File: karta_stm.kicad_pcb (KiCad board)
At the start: 2 copper layers, 99.1 x 63.5 mm, 130 parts, among them J1 Screw_Terminal_01x05, J2 Conn_01x06_Male, J3 Screw_Terminal_01x02, J4 Screw_Terminal_01x02, J5 Screw_Terminal_01x05, J6 Screw_Terminal_01x04, J7 Screw_Terminal_01x03, Q1 BC817, Q10 BC817, Q11 Q_PMOS_DGS, Q12 Q_NMOS_DGS, Q13 BC817, Q14 Q_PMOS_DGS, Q15 Q_NMOS_DGS, Q2 Q_PMOS_DGS, Q3 Q_NMOS_DGS, Q4 BC817, Q5 Q_PMOS_DGS, Q6 Q_NMOS_DGS, Q7 BC817, Q8 Q_PMOS_DGS, Q9 Q_NMOS_DGS, SW1 SW_Push, U1 STM32L4P5RET6, U10 EL817, U11 EL817, U12 EL817, U13 EL817, U2 MCP2562-H-SN, U3 LM2596S-5, U4 LD1117S33TR_SOT223, U5 MCP6001x-LT, U6 MCP6001x-LT, U7 MCP6001x-LT, U8 MCP6001x-LT, U9 MCP6001x-LT, Y1 16MHz

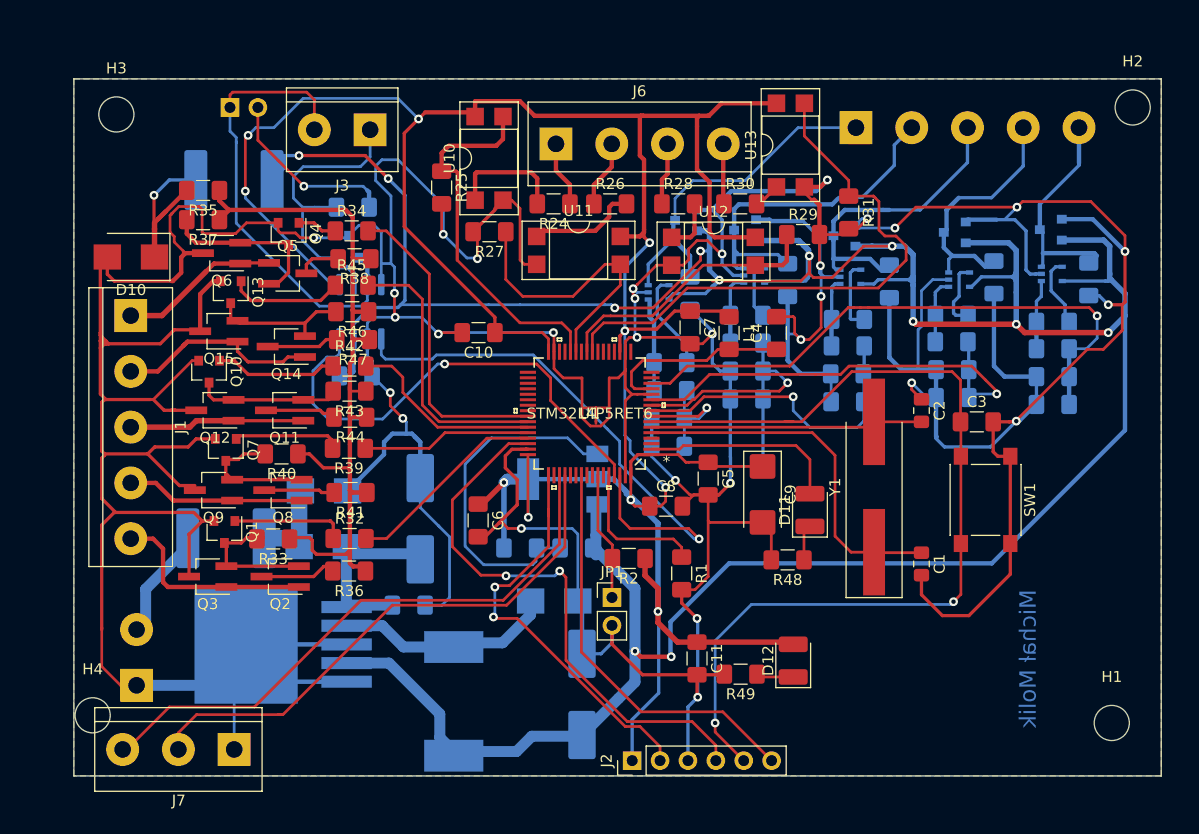
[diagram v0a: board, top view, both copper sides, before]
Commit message: Add files via upload
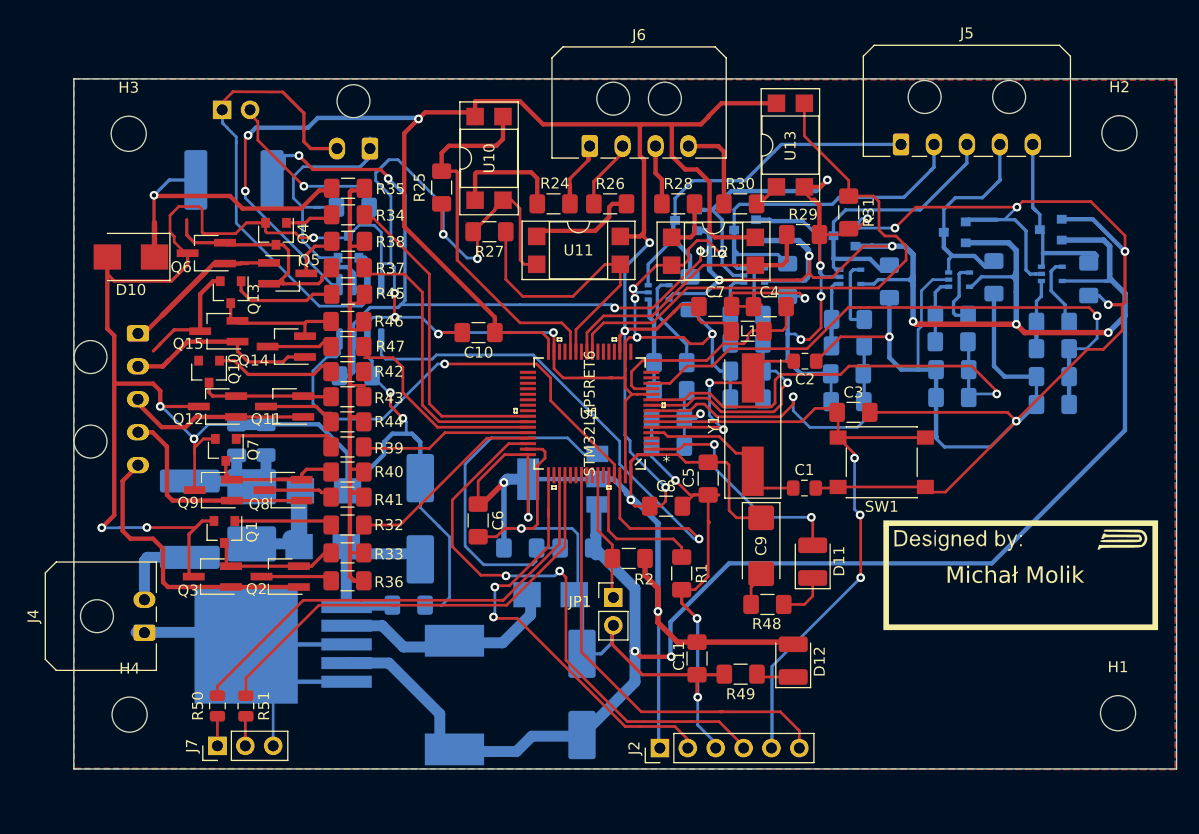
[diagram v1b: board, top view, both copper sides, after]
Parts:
- added C23: C, Capacitor_SMD:C_1206_3216Metric, B.Cu at (106.4, 84.9)
- added C24: C, Capacitor_SMD:C_1206_3216Metric, B.Cu at (103.7, 85.0)
- added G***: LOGO, logs:PUTM_LOGO_35mm, B.Cu at (165.0, 100.2)
- added G***: LOGO, logs:SignatureBox25mm, F.Cu at (175.1, 97.3)
- added L3: L, Inductor_SMD:L_2816_7142Metric_Pad3.20x4.45mm_HandSolder, B.Cu at (105.1, 91.8)
- added R50: R, Resistor_SMD:R_0805_2012Metric, F.Cu at (102.0, 109.2)
- added R51: R, Resistor_SMD:R_0805_2012Metric, F.Cu at (104.6, 109.2)
- J1: value Screw_Terminal_01x05 -> Conn_01x02_Female; footprint TerminalBlock:TerminalBlock_bornier-5_P5.08mm -> Connector_Molex:Molex_Micro-Fit_3.0_43650-0200_1x02_P3.00mm_Horizontal; moved to B.Cu
- J3: value Screw_Terminal_01x02 -> Conn_01x05_Female; footprint TerminalBlock:TerminalBlock_bornier-2_P5.08mm -> Connector_Molex:Molex_Micro-Fit_3.0_43650-0500_1x05_P3.00mm_Horizontal; moved to B.Cu
- J4: value Screw_Terminal_01x02 -> Conn_01x02_Female; footprint TerminalBlock:TerminalBlock_bornier-2_P5.08mm -> Connector_Molex:Molex_Micro-Fit_3.0_43650-0200_1x02_P3.00mm_Horizontal; moved to F.Cu
- J5: value Screw_Terminal_01x05 -> Conn_01x05_Female; footprint TerminalBlock:TerminalBlock_bornier-5_P5.08mm -> Connector_Molex:Molex_Micro-Fit_3.0_43650-0500_1x05_P3.00mm_Horizontal; moved to F.Cu
- J6: value Screw_Terminal_01x04 -> Conn_01x04_Female; footprint TerminalBlock:TerminalBlock_bornier-4_P5.08mm -> Connector_Molex:Molex_Micro-Fit_3.0_43650-0400_1x04_P3.00mm_Horizontal
- J7: value Screw_Terminal_01x03 -> Conn_01x03_Male; footprint TerminalBlock:TerminalBlock_bornier-3_P5.08mm -> Connector_PinHeader_2.54mm:PinHeader_1x03_P2.54mm_Vertical
- Y1: footprint Crystal:Crystal_SMD_HC49-SD_HandSoldering -> Crystal:Crystal_SMD_HC49-SD
- moved J3 28.1 mm to (94.7, 75.3), turned to 270 degrees
- moved J1 26.6 mm to (115.9, 58.4), turned to 180 degrees
- moved R37 13.9 mm to (113.9, 69.3)
- moved R35 13.2 mm to (113.9, 62.0)
- moved C1 12.7 mm to (155.5, 89.3), turned to 0 degrees
- moved Y1 12.4 mm to (150.7, 83.6)
- moved C2 11.5 mm to (155.5, 77.8), turned to 180 degrees
- moved C3 11.3 mm to (159.9, 82.4)
- moved SW1 10.1 mm to (162.5, 87.0), turned to 180 degrees
- moved R33 6.89 mm to (113.8, 95.2)
- moved R40 6.23 mm to (113.8, 87.9)
- moved J4 4.85 mm to (95.3, 102.5)
- moved D11 4.71 mm to (156.2, 96.0)
- moved C9 4.68 mm to (151.5, 94.6)
- moved R48 4.46 mm to (152.1, 99.9)
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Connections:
- F1 pad 1: Net-(D2-Pad1) -> Net-(C23-Pad1)
- J1 pad 1: OUT_4 -> CAN_L
- J1 pad 2: OUT_3 -> CAN_H
- J3 pad 1: CAN_L -> OUT_4
- J3 pad 2: CAN_H -> OUT_3
- J7 pad 1: GND -> Net-(J7-Pad1)
- J7 pad 2: UART_RX -> Net-(J7-Pad2)
- J7 pad 3: UART_TX -> GND
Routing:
- net NRST: track 86.8 -> 60.4 mm, vias 2 -> 3
- net +5VD: track 69.5 -> 49.4 mm
- net +3V3: track 268.7 -> 286.5 mm
- net OSC_IN: track 33.4 -> 15.9 mm
- net GND: track 728.7 -> 711.5 mm, vias 30 -> 34
- net Net-(C23-Pad1): track 0.00 -> 12.7 mm
- net Net-(D10-Pad1): track 15.7 -> 28.0 mm
- net UART_TX: track 53.8 -> 43.7 mm
- net UART_RX: track 50.6 -> 42.5 mm
- net ADC_IN3: track 32.4 -> 40.4 mm
- net OUT_0: track 18.9 -> 26.5 mm
- net Net-(Q4-Pad3): track 15.8 -> 22.5 mm
- net ADC_3: track 27.4 -> 22.9 mm
- net OSC_OUT: track 24.8 -> 20.8 mm, vias 0 -> 2
- net Net-(C4-Pad1): track 17.3 -> 21.3 mm
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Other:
- board size 99.1 x 63.5 mm -> 100.5 x 62.9 mm
